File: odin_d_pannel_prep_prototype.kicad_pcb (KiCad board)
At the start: 2 copper layers, 27 parts, among them J1 Conn_01x03, Q4 Q_NPN_BEC, Q5 Q_NPN_BEC, T1 BT136S

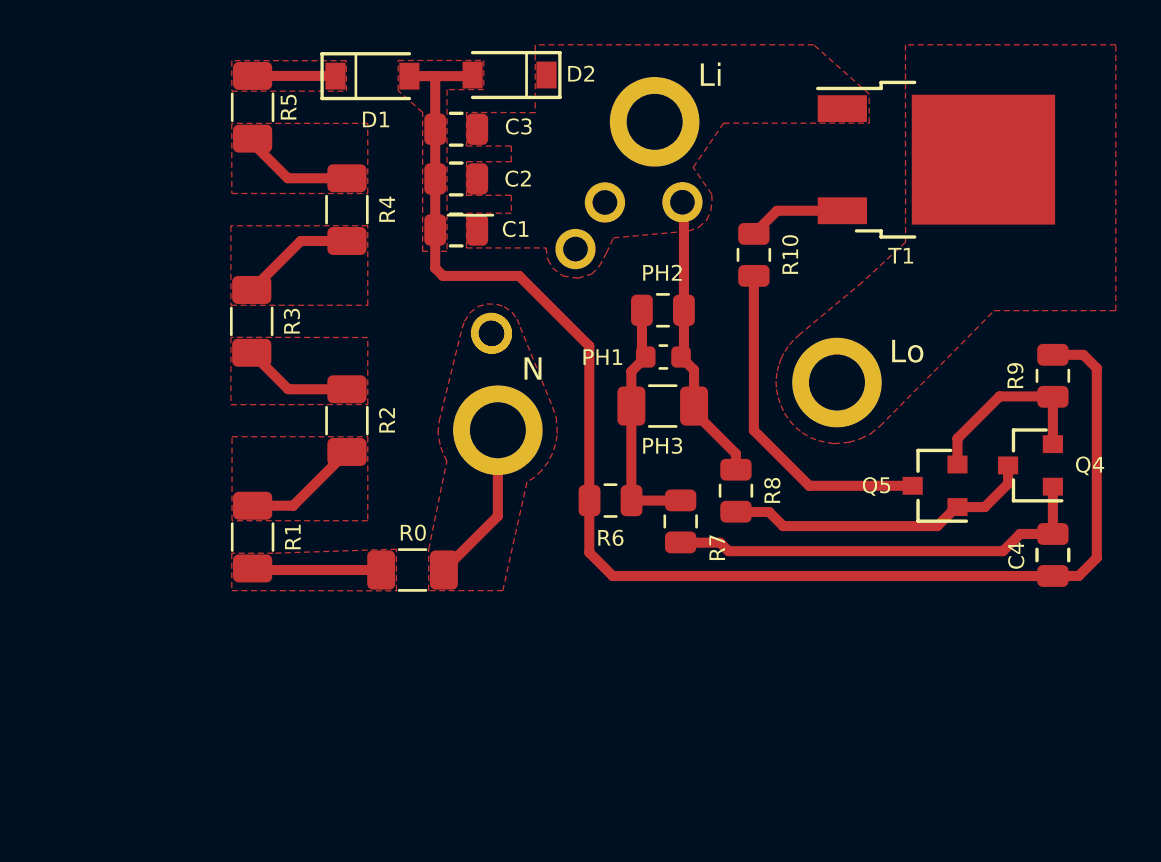
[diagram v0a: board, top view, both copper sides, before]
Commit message: Added files for production run
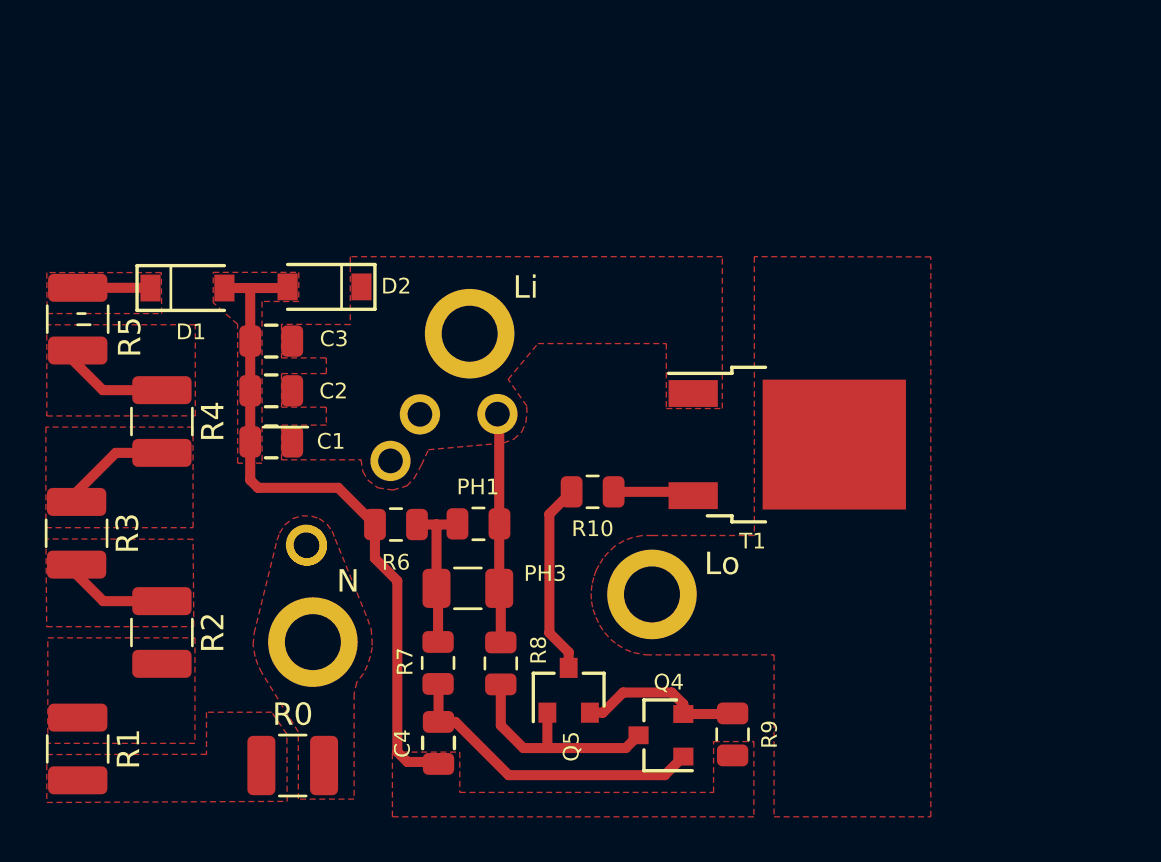
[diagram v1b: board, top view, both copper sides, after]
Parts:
- removed the PH1 at (149.0, 90.8)
- R0, R1, R2, R3, R4, R5: value 5.6k -> 3k; footprint Resistor_SMD:R_1206_3216Metric -> Resistor_SMD:R_1210_3225Metric
- moved C4 28.7 mm to (139.0, 108.0)
- moved R9 21.5 mm to (152.1, 107.7), turned to 270 degrees
- moved Q4 20.4 mm to (148.9, 107.7)
- moved Q5 18.7 mm to (144.8, 105.7), turned to 90 degrees
- moved T1 14.4 mm to (154.5, 94.7)
- moved R8 13.0 mm to (141.7, 104.5)
- moved R10 12.8 mm to (145.8, 96.8), turned to 180 degrees
- moved PH1 12.6 mm to (140.7, 98.3)
- moved J1 12.6 mm to (140.3, 98.4)
- moved D1 12.6 mm to (127.8, 87.7)
- moved D2 12.6 mm to (133.9, 87.7)
- moved RV1 12.6 mm to (138.1, 93.4)
- moved RV2 12.6 mm to (136.8, 95.5)
- moved R2 12.6 mm to (126.6, 103.1)
- moved R4 12.6 mm to (126.6, 93.7)
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- renumbered PH2 to PH1
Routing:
- net /GND: track 63.5 -> 30.4 mm
- net /NEUTRAL: track 8.14 -> 0.00 mm
- net Net-(Q5-Pad3): track 15.0 -> 8.63 mm
- net Net-(R0-Pad1): track 5.77 -> 0.00 mm
- net Net-(C4-Pad1): track 19.5 -> 14.0 mm
- net Net-(R1-Pad1): track 5.20 -> 0.00 mm
- net Net-(PH1-Pad1): track 11.3 -> 7.10 mm
- net Net-(Q4-Pad3): track 14.0 -> 10.3 mm
- net /LIVE: track 13.8 -> 11.4 mm
- net Net-(Q4-Pad2): track 8.32 -> 7.41 mm
- net Net-(R10-Pad1): track 4.38 -> 3.62 mm
